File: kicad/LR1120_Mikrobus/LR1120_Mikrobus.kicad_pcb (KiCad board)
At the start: 4 copper layers, 57.2 x 25.4 mm, 110 parts, among them CON1 MIKROBUS_MODULE_CONN, J1 Conn_01x07, J2 Conn_01x07, Q1 NX2016SA-32M-EXS00A-CS06465, Q2 NT2016SA-32M-END4263A, Q3 NX3215SA, U1 LR1120, U2 SKY13588-460LF, U5 LIS2DE12, U7 M24128-BFMH6TG, U8 BGA524N6E6327XTSA1

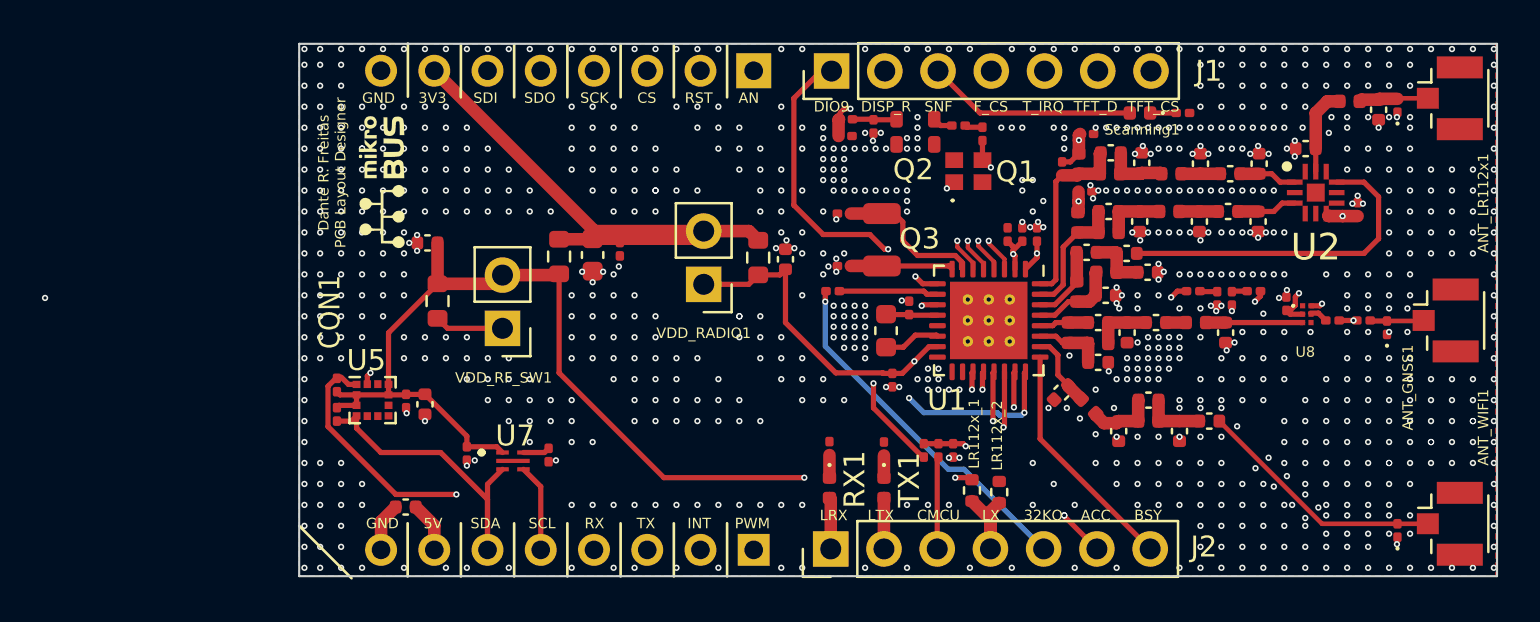
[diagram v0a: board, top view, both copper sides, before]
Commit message: gerbers generated
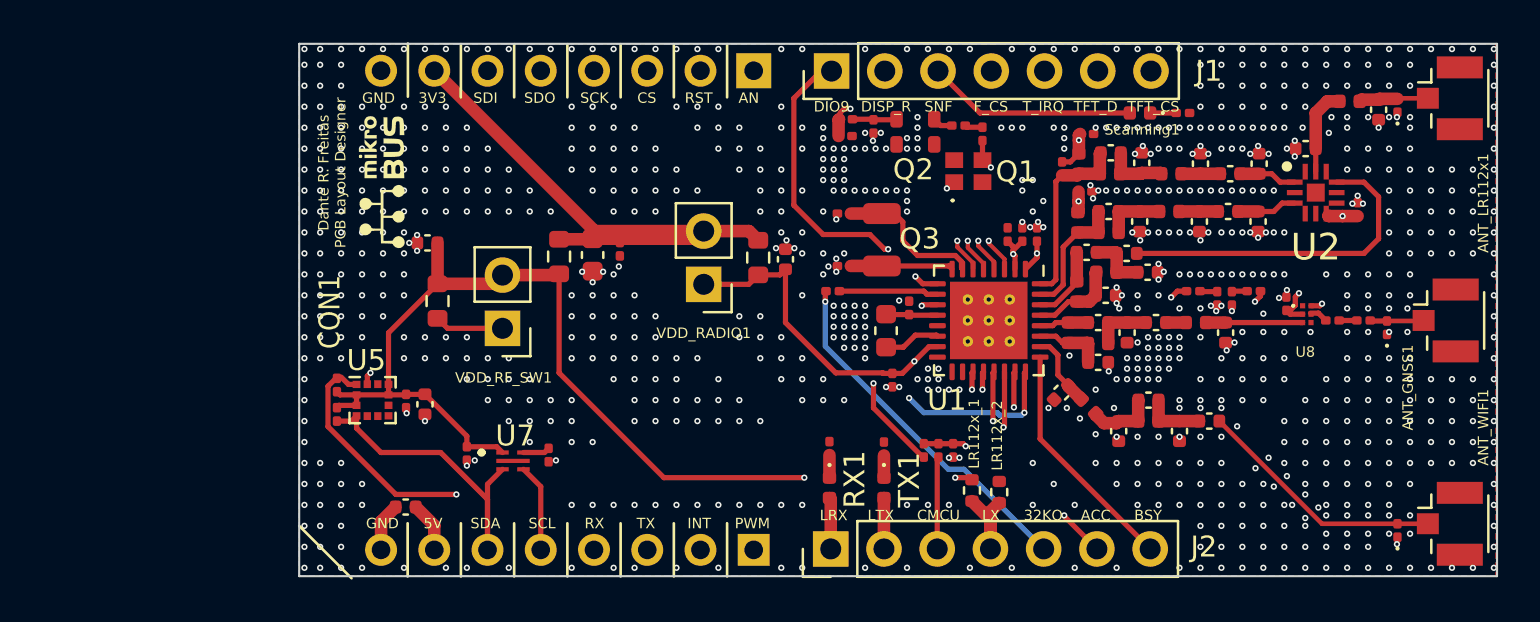
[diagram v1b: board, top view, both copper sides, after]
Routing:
- net Net-(C54-Pad2): vias 1 -> 0
- net GND: vias 881 -> 875
- net /ACC_INT1: vias 3 -> 2
- net (no net): vias 1 -> 0
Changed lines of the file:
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@@
       (outputformat 1)
       (mirror false)
-      (drillshape 1)
+      (drillshape 0)
       (scaleselection 1)
-      (outputdirectory "")
+      (outputdirectory "../../gerber/")
     )
   )
@@
     (fp_line (start 2.5 -2.5) (end 2.5 2.5) (layer "F.Fab") (width 0.1))
     (fp_line (start -2.5 2.5) (end -2.5 -1.5) (layer "F.Fab") (width 0.1))
-    (pad "" smd roundrect locked (at 0.5 0.5 270) (size 0.806226 0.806226) (layers "F.Paste") (roundrect_rratio 0.25))
+    (pad "" smd roundrect locked (at 0.5 0.5 270) (size 0.806226 0.806226) (layers "F.Paste") (roundrect_rratio 0.2500006202))
     (pad "" smd custom locked (at 1.425 1.425 270) (size 0.601758 0.601758) (layers "F.Paste")
       (options (clearance outline) (anchor circle))
@@
           ) (width 0.146515) (fill yes))
       ))
-    (pad "" smd roundrect locked (at 0.5 -0.5 270) (size 0.806226 0.806226) (layers "F.Paste") (roundrect_rratio 0.25))
-    (pad "" smd roundrect locked (at -0.5 0.5 270) (size 0.806226 0.806226) (layers "F.Paste") (roundrect_rratio 0.25))
+    (pad "" smd roundrect locked (at 0.5 -0.5 270) (size 0.806226 0.806226) (layers "F.Paste") (roundrect_rratio 0.2500006202))
+    (pad "" smd roundrect locked (at -0.5 0.5 270) (size 0.806226 0.806226) (layers "F.Paste") (roundrect_rratio 0.2500006202))
     (pad "" smd custom locked (at 1.425 0.5 270) (size 0.612035 0.612035) (layers "F.Paste")
       (options (clearance outline) (anchor circle))
@@
           ) (width 0.146515) (fill yes))
       ))
-    (pad "" smd roundrect locked (at -0.5 -0.5 270) (size 0.806226 0.806226) (layers "F.Paste") (roundrect_rratio 0.25))
+    (pad "" smd roundrect locked (at -0.5 -0.5 270) (size 0.806226 0.806226) (layers "F.Paste") (roundrect_rratio 0.2500006202))
     (pad "1" smd roundrect locked (at -2.45 -1.75 270) (size 0.8 0.25) (layers "F.Cu" "F.Paste" "F.Mask") (roundrect_rratio 0.25)
       (net 7 "/VR_PA") (pinfunction "VR_PA") (pintype "output"))
@@
     (effects (font (size 0.5 0.5) (thickness 0.05)))
   )
-  (dimension (type aligned) (layer "F.SilkS")
-    (pts (xy 100 125.4) (xy 100 100))
-    (height -2)
-    (gr_text "25.4000 mm" (at 97.375 112.7 90) (layer "F.SilkS")
-      (effects (font (size 0.5 0.5) (thickness 0.15)))
-    )
-    (format (units 3) (units_format 1) (precision 4))
-    (style (thickness 0.125) (arrow_length 1.27) (text_position_mode 0) (extension_height 0.58642) (extension_offset 0.5) keep_text_aligned)
-  )
-  (dimension (type aligned) (layer "F.SilkS")
-    (pts (xy 100 125.4) (xy 157.15 125.4))
-    (height 3.1)
-    (gr_text "57.1500 mm" (at 128.575 127.875) (layer "F.SilkS")
-      (effects (font (size 0.5 0.5) (thickness 0.15)))
-    )
-    (format (units 3) (units_format 1) (precision 4))
-    (style (thickness 0.125) (arrow_length 1.27) (text_position_mode 0) (extension_height 0.58642) (extension_offset 0.5) keep_text_aligned)
-  )
-  (via (at 87.875 112.125) (size 0.3) (drill 0.15) (layers "F.Cu" "B.Cu") (free) (net 0))
   (segment (start 151.9 113.225) (end 153.625 113.225) (width 0.22) (layer "F.Cu") (net 1))
   (segment (start 151.125 113.225) (end 151.1 113.2) (width 0.25) (layer "F.Cu") (net 1))
@@
   (via (at 149 117) (size 0.3) (drill 0.15) (layers "F.Cu" "B.Cu") (free) (net 2))
   (via (at 156 118) (size 0.3) (drill 0.15) (layers "F.Cu" "B.Cu") (free) (net 2))
-  (via (at 152 120) (size 0.3) (drill 0.15) (layers "F.Cu" "B.Cu") (free) (net 2))
   (via (at 142 104) (size 0.3) (drill 0.15) (layers "F.Cu" "B.Cu") (free) (net 2))
   (via (at 125 105.5) (size 0.3) (drill 0.15) (layers "F.Cu" "B.Cu") (free) (net 2))
@@
   (via (at 134.5 106.5) (size 0.3) (drill 0.15) (layers "F.Cu" "B.Cu") (free) (net 2))
   (via (at 144 101) (size 0.3) (drill 0.15) (layers "F.Cu" "B.Cu") (free) (net 2))
-  (via (at 103 105) (size 0.3) (drill 0.15) (layers "F.Cu" "B.Cu") (free) (net 2))
   (via (at 144.5 107) (size 0.3) (drill 0.15) (layers "F.Cu" "B.Cu") (free) (net 2))
   (via (at 114 106) (size 0.3) (drill 0.15) (layers "F.Cu" "B.Cu") (free) (net 2))
@@
   (via (at 141.5 109) (size 0.3) (drill 0.15) (layers "F.Cu" "B.Cu") (free) (net 2))
   (via (at 153 121) (size 0.3) (drill 0.15) (layers "F.Cu" "B.Cu") (free) (net 2))
-  (via (at 156 118) (size 0.3) (drill 0.15) (layers "F.Cu" "B.Cu") (free) (net 2))
   (via (at 103 122) (size 0.3) (drill 0.15) (layers "F.Cu" "B.Cu") (free) (net 2))
   (via (at 102 121) (size 0.3) (drill 0.15) (layers "F.Cu" "B.Cu") (free) (net 2))
@@
   (via (at 132 125) (size 0.3) (drill 0.15) (layers "F.Cu" "B.Cu") (free) (net 2))
   (via (at 114 103) (size 0.3) (drill 0.15) (layers "F.Cu" "B.Cu") (free) (net 2))
-  (via (at 121 113) (size 0.3) (drill 0.15) (layers "F.Cu" "B.Cu") (free) (net 2))
   (via (at 139.25 112) (size 0.3) (drill 0.15) (layers "F.Cu" "B.Cu") (free) (net 2))
   (via (at 125 104) (size 0.3) (drill 0.15) (layers "F.Cu" "B.Cu") (free) (net 2))
@@
   (via (at 155 116) (size 0.3) (drill 0.15) (layers "F.Cu" "B.Cu") (free) (net 2))
   (via (at 101 113) (size 0.3) (drill 0.15) (layers "F.Cu" "B.Cu") (free) (net 2))
-  (via (at 128.75 112.25) (size 0.3) (drill 0.15) (layers "F.Cu" "B.Cu") (free) (net 2))
+  (via (at 128.625 112.25) (size 0.3) (drill 0.15) (layers "F.Cu" "B.Cu") (free) (net 2))
   (via (at 150.75 107.625) (size 0.3) (drill 0.15) (layers "F.Cu" "B.Cu") (free) (net 2))
   (via (at 104 108) (size 0.3) (drill 0.15) (layers "F.Cu" "B.Cu") (free) (net 2))
@@
   (via (at 157 123) (size 0.3) (drill 0.15) (layers "F.Cu" "B.Cu") (free) (net 2))
   (via (at 127 100.25) (size 0.3) (drill 0.15) (layers "F.Cu" "B.Cu") (free) (net 2))
-  (via (at 154 119) (size 0.3) (drill 0.15) (layers "F.Cu" "B.Cu") (free) (net 2))
   (via (at 144 125) (size 0.3) (drill 0.15) (layers "F.Cu" "B.Cu") (free) (net 2))
   (via (at 117 117) (size 0.3) (drill 0.15) (layers "F.Cu" "B.Cu") (free) (net 2))
@@
   (via (at 102 100.25) (size 0.3) (drill 0.15) (layers "F.Cu" "B.Cu") (free) (net 2))
   (via (at 143 118.75) (size 0.3) (drill 0.15) (layers "F.Cu" "B.Cu") (free) (net 2))
-  (via (at 117 107) (size 0.3) (drill 0.15) (layers "F.Cu" "B.Cu") (free) (net 2))
   (via (at 145 104) (size 0.3) (drill 0.15) (layers "F.Cu" "B.Cu") (free) (net 2))
   (via (at 111 119) (size 0.3) (drill 0.15) (layers "F.Cu" "B.Cu") (free) (net 2))
@@
   (segment (start 150.3 113.2) (end 149.62 113.2) (width 0.25) (layer "F.Cu") (net 39))
   (segment (start 150.46 113.2) (end 150.3 113.2) (width 0.25) (layer "F.Cu") (net 39))
-  (via (at 150.3 113.2) (size 0.3) (drill 0.15) (layers "F.Cu" "B.Cu") (net 39))
   (segment (start 125.735 103.625) (end 125.76 103.6) (width 0.6) (layer "F.Cu") (net 40))
   (segment (start 132.9 109.4) (end 132.9 109.519264) (width 0.2) (layer "F.Cu") (net 40))
@@
   (via (at 103.4 115.7) (size 0.3) (drill 0.15) (layers "F.Cu" "B.Cu") (net 55))
   (via (at 136.5 122.5) (size 0.3) (drill 0.15) (layers "F.Cu" "B.Cu") (net 55))
-  (via (at 136.5 122.5) (size 0.3) (drill 0.15) (layers "F.Cu" "B.Cu") (net 55))
   (segment (start 106.5 115.7) (end 103.4 115.7) (width 0.25) (layer "In2.Cu") (net 55))
